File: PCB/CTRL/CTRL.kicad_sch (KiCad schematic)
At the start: 45 parts, among them IC1 TMP112NAIDRLR, IC2 LTC4311CSC6#TRPBF, J1 Conn_02x06_Odd_Even, J2 Conn_02x06_Odd_Even, J4 Conn_01x04_Pin, J5 RESET, J6 Conn_01x04_Pin, U1 MB85RS2MT, U2 ATSAMD21G18A-A, U3 MAX6372, U4 SN65220DBVR, Y1 8MHz

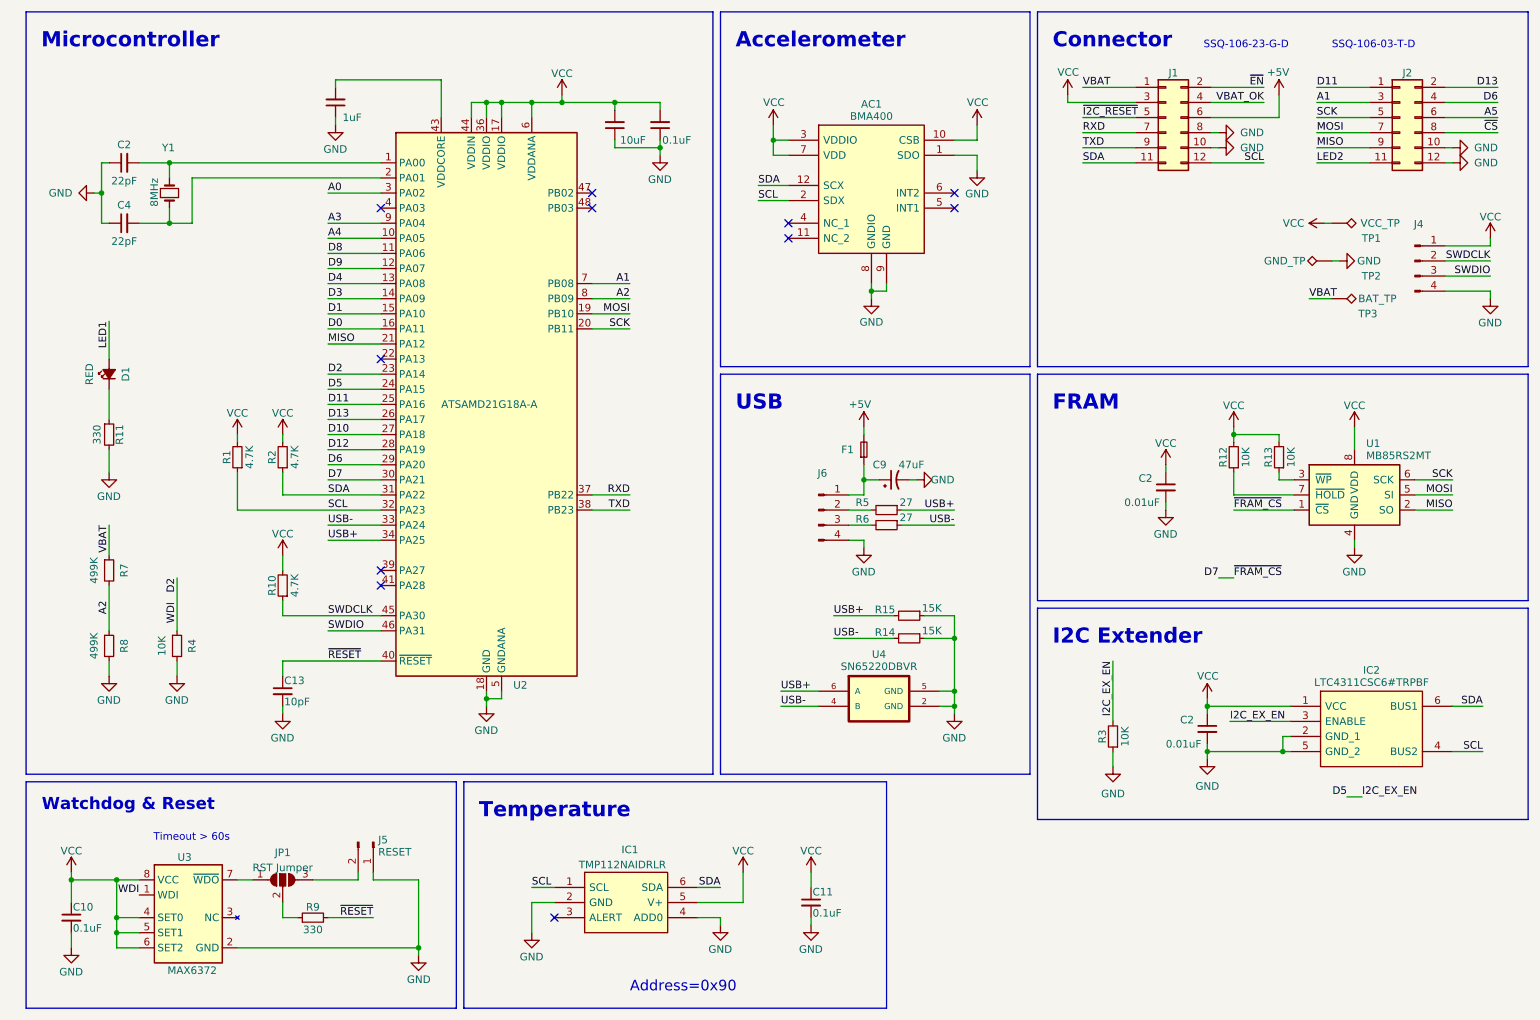
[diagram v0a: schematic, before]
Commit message: udated by FZ
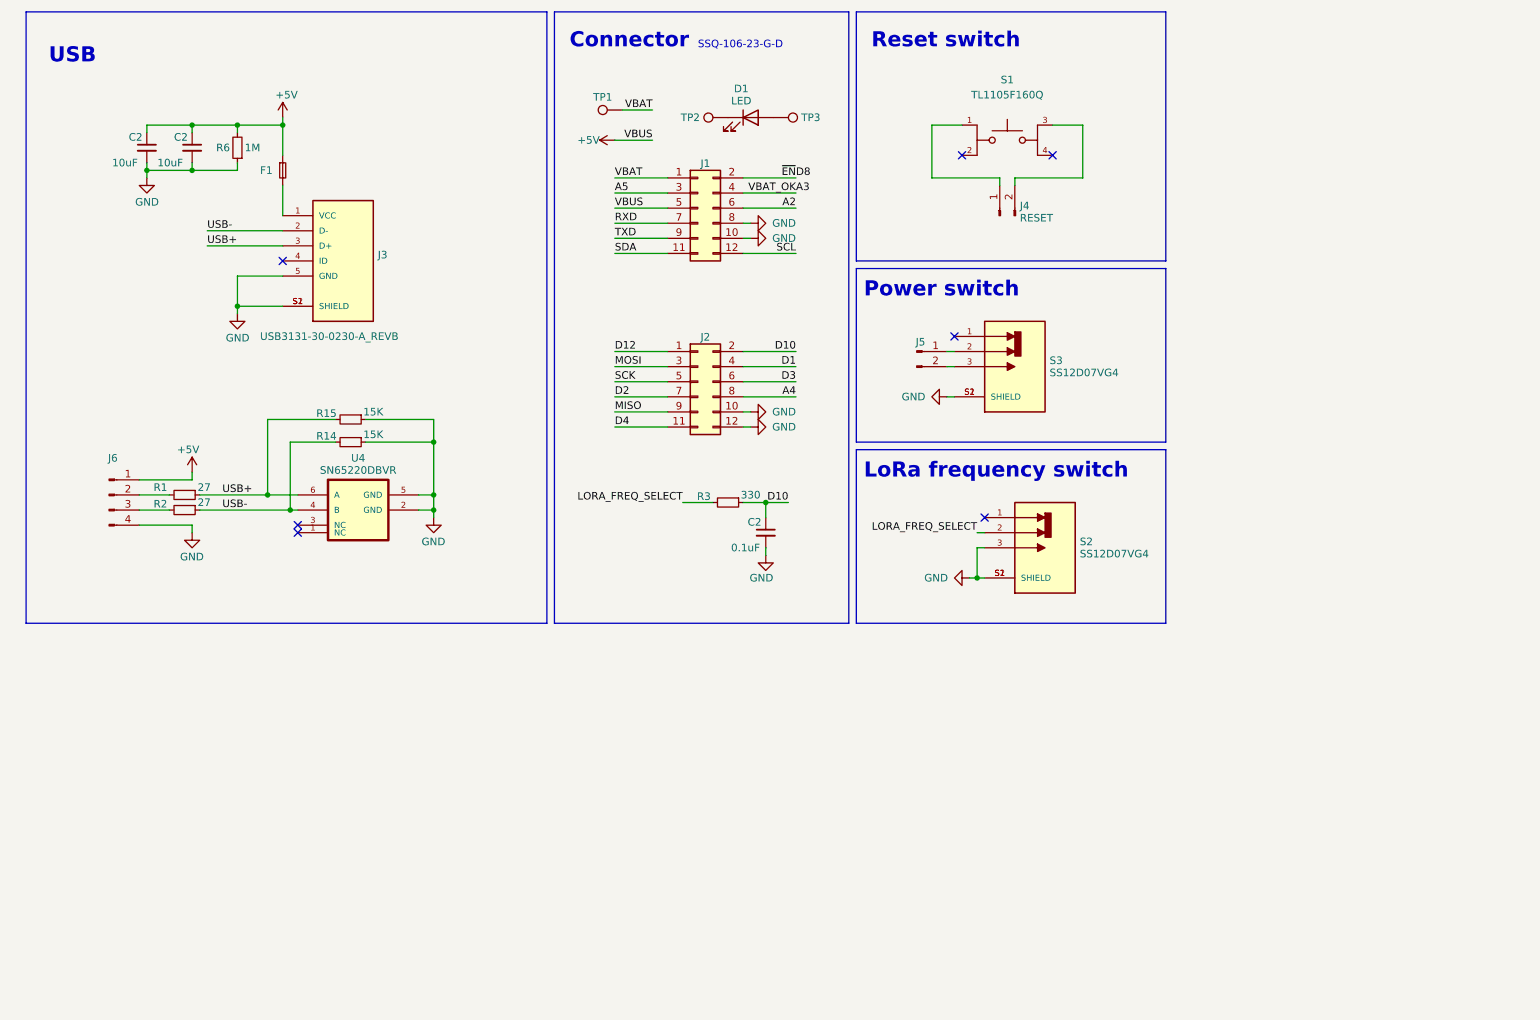
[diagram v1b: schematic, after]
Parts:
- removed AC1: BMA400, SamacSys_Parts:BOSCH_LGA-12, symbol SamacSys_Parts:BMA400
- removed C10, C11: 0.1uF, Capacitor_SMD:C_0402_1005Metric, symbol Device:C_Small
- removed C12: 1uF, Capacitor_SMD:C_0402_1005Metric_Pad0.74x0.62mm_HandSolder, symbol Device:C_Small
- removed C13: 10pF, Capacitor_SMD:C_0402_1005Metric, symbol Device:C_Small
- removed C2 (x2): 0.01uF, Capacitor_SMD:C_1206_3216Metric_Pad1.33x1.80mm_HandSolder, symbol Device:C_Small
- removed C2, C4: 22pF, Capacitor_SMD:C_0402_1005Metric_Pad0.74x0.62mm_HandSolder, symbol Device:C_Small
- removed C5: 10uF, Capacitor_SMD:C_0402_1005Metric_Pad0.74x0.62mm_HandSolder, symbol Device:C_Small
- removed C6: 0.1uF, Capacitor_SMD:C_0402_1005Metric_Pad0.74x0.62mm_HandSolder, symbol Device:C_Small
- removed C9: 47uF, Capacitor_SMD:C_0805_2012Metric_Pad1.18x1.45mm_HandSolder, symbol Device:C_Polarized_Small_US
- removed D1: RED, LED_SMD:LED_0603_1608Metric_Pad1.05x0.95mm_HandSolder, symbol Device:LED_Small_Filled
- removed IC1: TMP112NAIDRLR, Mylib:SOT50P160X60-6N, symbol SamacSys_Parts:TMP112NAIDRLR
- removed IC2: LTC4311CSC6#TRPBF, SamacSys_Parts:SOT65P210X100-6N, symbol SamacSys_Parts:LTC4311CSC6#TRPBF
- removed J4: Conn_01x04_Pin, symbol Connector:Conn_01x04_Pin
- removed JP1: RST Jumper, Jumper:SolderJumper-3_P1.3mm_Open_RoundedPad1.0x1.5mm, symbol Jumper:SolderJumper_3_Open
- removed R10: 4.7K, Resistor_SMD:R_0402_1005Metric_Pad0.72x0.64mm_HandSolder, symbol Device:R_Small
- removed R11, R9: 330, Resistor_SMD:R_0402_1005Metric_Pad0.72x0.64mm_HandSolder, symbol Device:R_Small
- removed R12, R13: 10K, Resistor_SMD:R_0402_1005Metric_Pad0.72x0.64mm_HandSolder, symbol Device:R_Small
- removed R4: 10K, Resistor_SMD:R_0402_1005Metric, symbol Device:R_Small
- removed R5: 27, Resistor_SMD:R_0402_1005Metric_Pad0.72x0.64mm_HandSolder, symbol Device:R_Small
- removed R7, R8: 499K, Resistor_SMD:R_0402_1005Metric_Pad0.72x0.64mm_HandSolder, symbol Device:R_Small
- removed TP1: VCC_TP, TestPoint:TestPoint_Pad_1.5x1.5mm, symbol Connector:TestPoint_Alt
- removed TP2: GND_TP, TestPoint:TestPoint_Pad_1.5x1.5mm, symbol Connector:TestPoint_Alt
- removed TP3: BAT_TP, TestPoint:TestPoint_Pad_1.0x1.0mm, symbol Connector:TestPoint_Alt
- removed U1: MB85RS2MT, symbol Memory_NVRAM:MB85RS2MT
- removed U2: ATSAMD21G18A-A, Package_QFP:TQFP-48_7x7mm_P0.5mm, symbol MCU_Microchip_SAMD:ATSAMD21G18A-A
- removed U3: MAX6372, Package_TO_SOT_SMD:SOT-23-8, symbol Power_Supervisor:MAX6372
- removed Y1: 8MHz, Capacitor_SMD:C_0805_2012Metric_Pad1.18x1.45mm_HandSolder, symbol Device:Crystal_Small
- added C2 (x2): 10uF, Capacitor_SMD:C_1206_3216Metric_Pad1.33x1.80mm_HandSolder, symbol Device:C_Small
- added C2: 0.1uF, Capacitor_SMD:C_0402_1005Metric_Pad0.74x0.62mm_HandSolder, symbol Device:C_Small
- added D1: LED, Diode_SMD:D_0603_1608Metric_Pad1.05x0.95mm_HandSolder, symbol Device:LED
- added J3: USB3131-30-0230-A_REVB, Mylib:GCT_USB3131-30-0230-A_REVB, symbol USB3131-30-0230-A_REVB:USB3131-30-0230-A_REVB
- added J4: RESET, Connector_PinHeader_2.00mm:PinHeader_1x02_P2.00mm_Vertical, symbol Connector:Conn_01x02_Pin
- added S1: TL1105F160Q, Mylib:SW_TL1105F160Q, symbol TL1105F160Q:TL1105F160Q
- added S2, S3: SS12D07VG4, Mylib:SW_SS12D07VG4, symbol SS12D07VG4:SS12D07VG4
- added TP1, TP2, TP3: TestPoint, TestPoint:TestPoint_Pad_1.5x1.5mm, symbol Connector:TestPoint
- F1: footprint (none) -> Fuse:Fuse_1206_3216Metric_Pad1.42x1.75mm_HandSolder
- J5: footprint (none) -> Connector_PinHeader_2.00mm:PinHeader_1x02_P2.00mm_Vertical
- J6: footprint (none) -> Connector_PinHeader_2.00mm:PinHeader_1x04_P2.00mm_Vertical
- R1, R2: value 4.7K -> 27
- R3: value 10K -> 330
- R6: value 27 -> 1M; footprint Resistor_SMD:R_0402_1005Metric_Pad0.72x0.64mm_HandSolder -> Resistor_SMD:R_0603_1608Metric_Pad0.98x0.95mm_HandSolder
- U4: footprint SN65220DBVR:SOT95P280X145-6N -> SamacSys_Parts:SOT95P275X135-6N
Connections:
- net A1 is gone; now on net MOSI: J2.3 (Pin_3)
- net D11 is gone; now on net D12: J2.1 (Pin_1)
- net D13 is gone; now on net D10: J2.2 (Pin_2)
- net D6 is gone; now on net D1: J2.4 (Pin_4)
- net LED2 is gone; now on net D4: J2.11 (Pin_11)
- net VBAT_OK is gone; now on net A3: J1.4 (Pin_4)
- net ~{CS} is gone; now on net A4: J2.8 (Pin_8)
- net ~{EN} is gone; now on net D8: J1.2 (Pin_2)
- net ~{I2C_RESET} is gone; now on net +5V: J1.5 (Pin_5)
- net +5V: now also F1.1, J6.1 (Pin_1), R6.2, C2.1, C2.1; no longer F1.2, J1.6 (Pin_6)
- net A2: now also J1.6 (Pin_6)
- net A5: now also J1.3 (Pin_3); no longer J2.6 (Pin_6)
- net D10: now also R3.1, C2.1
- net D2: now also J2.7 (Pin_7)
- net D3: now also J2.6 (Pin_6)
- net GND: now also R6.1, C2.2, C2.2, C2.2, J3.5 (GND), J3.S1 (SHIELD), J3.S2 (SHIELD), S2.3, S2.S1 (SHIELD), S2.S2 (SHIELD), S3.S1 (SHIELD), S3.S2 (SHIELD); no longer J5.1 (Pin_1), R3.1
- net MOSI: no longer J2.7 (Pin_7)
- net SCL: no longer R1.1
- net SDA: no longer R2.1
- net USB+: now also R1.1, J3.3 (D+)
- net USB-: now also R2.1, J3.2 (D-); no longer R6.1
- net VBAT: now also TP1.1
- net at J6.2 (Pin_2): now also R1.2
- net at J5.2 (Pin_2): now also S3.3
- net at J6.3 (Pin_3): now also R2.2; no longer R6.2
- net D5 renamed LORA_FREQ_SELECT
- net LORA_FREQ_SELECT: now also S2.2
- removed net VCC: J1.3 (Pin_3), R1.2, R2.2
- new net: J5.1 (Pin_1), S3.2
- new net: D1.1 (K), TP2.1
- new net: D1.2 (A), TP3.1
- new net: F1.2, J3.1 (VCC)
- new net: J4.1 (Pin_1), S1.1
- new net: J4.2 (Pin_2), S1.3
- no-connect marks 11 -> 7
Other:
- note added: "LoRa frequency switch"
- note added: "Power switch"
- note added: "Reset switch"
- note removed: "Accelerometer"
- note removed: "Address=0x90"
- note removed: "FRAM"
- note removed: "I2C Extender"
- note removed: "Microcontroller"
- note removed: "SSQ-106-03-T-D"
- note removed: "Temperature"
- note removed: "Timeout > 60s"
- note removed: "Watchdog & Reset"
- moved on the sheet: F1, J1, J2, J6, R14, R15
